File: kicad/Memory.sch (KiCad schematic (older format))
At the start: 0 parts

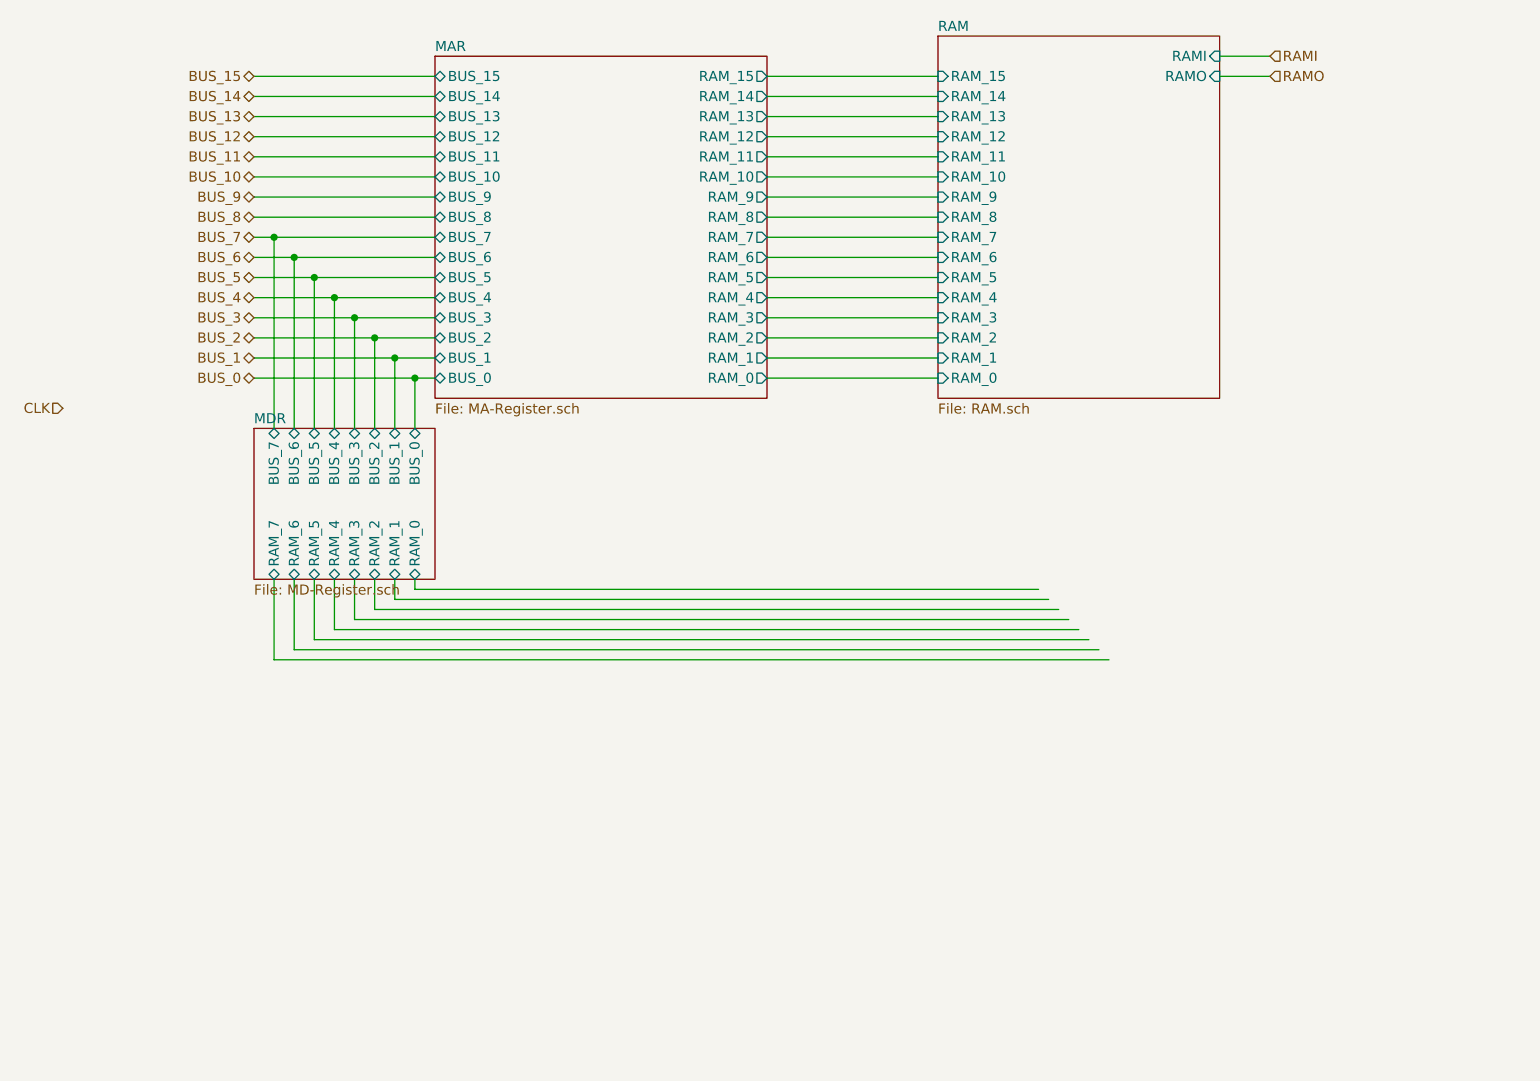
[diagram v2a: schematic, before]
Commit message: Finish todo list
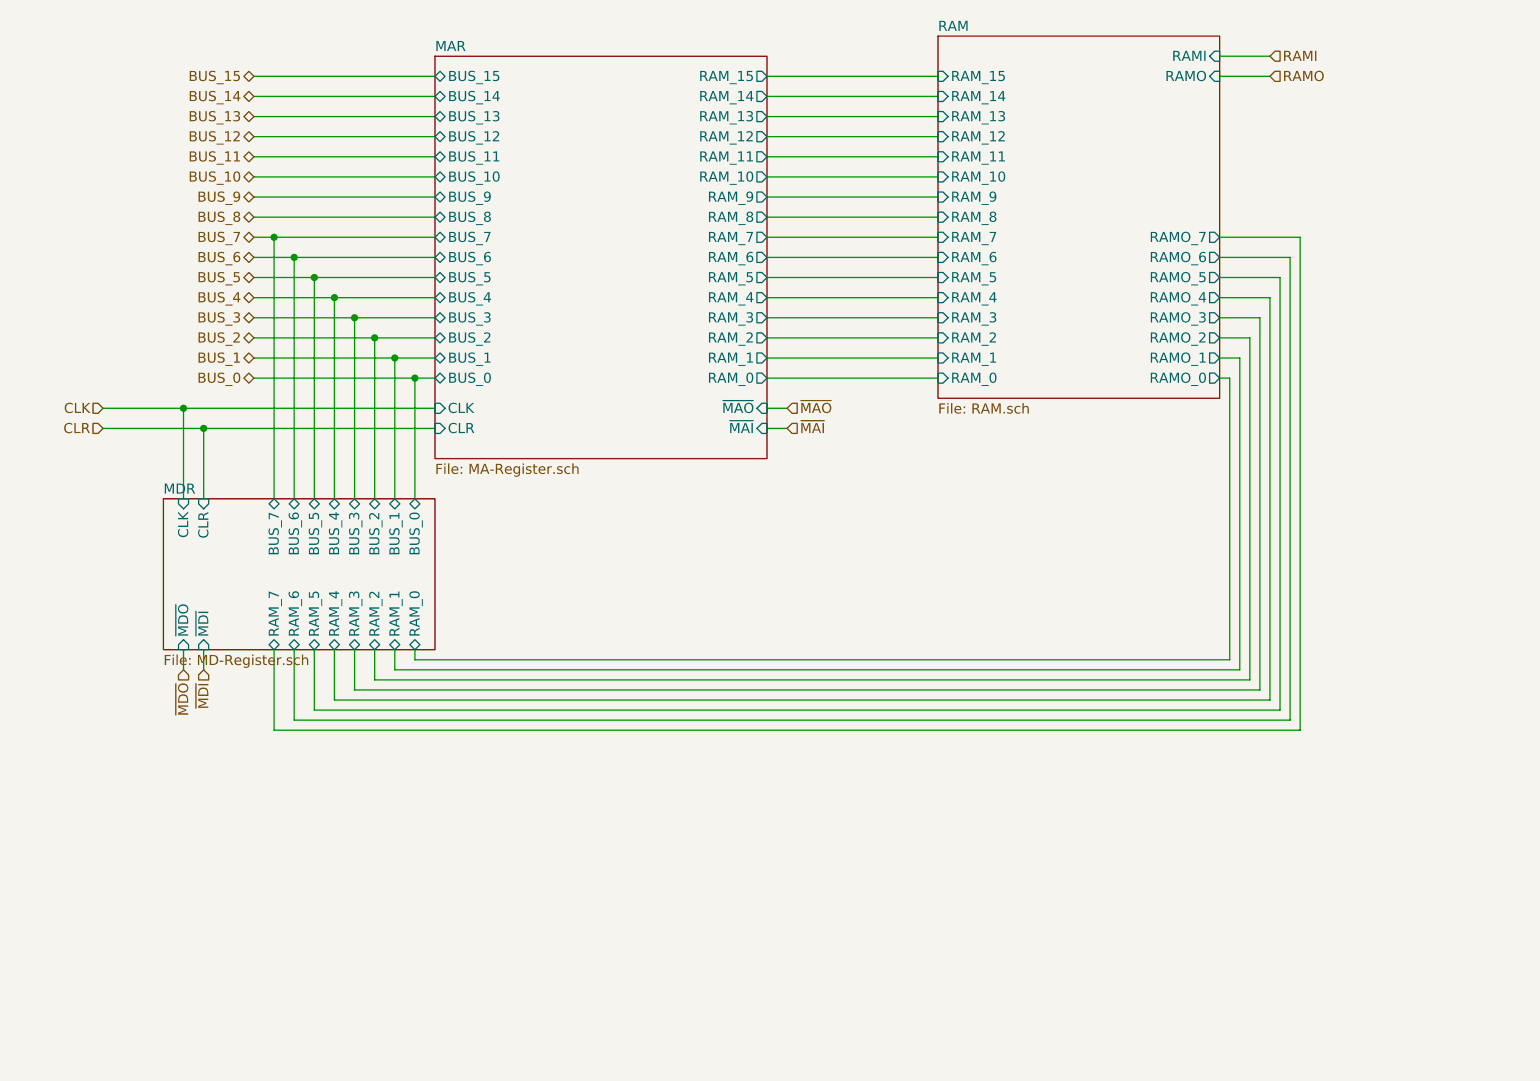
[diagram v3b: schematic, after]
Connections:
- net labels added: CLR, ~MAI~, ~MAO~, ~MDI~, ~MDO~
- wire segments 66 -> 92
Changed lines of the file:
@@
 $Descr USLetter 11000 8500
 encoding utf-8
-Sheet 13 26
+Sheet 14 26
 Title "Memory"
-Date "2019-09-26"
+Date "2019-10-03"
 Rev "v0.1"
 Comp "Christopher Milan"
@@
 Text HLabel 2050 950  0    50   BiDi ~ 0
 BUS_15
-Text HLabel 1100 2600 0    50   Input ~ 0
+Text HLabel 1300 2600 0    50   Input ~ 0
 CLK
 $Sheet
-S 2950 850  1650 1700
+S 2950 850  1650 2000
 U 5D807A05
 F0 "MAR" 50
@@
 F32 "RAM_14" O R 4600 1050 50
 F33 "RAM_15" O R 4600 950 50
+F34 "CLK" I L 2950 2600 50
+F35 "~MAO~" I R 4600 2600 50
+F36 "~MAI~" I R 4600 2700 50
+F37 "CLR" I L 2950 2700 50
 $EndSheet
 Wire Wire Line
@@
 	2050 2350 2750 2350
 Wire Wire Line
-	2850 2700 2850 2450
+	2850 3050 2850 2450
 Connection ~ 2850 2450
 Wire Wire Line
 	2850 2450 2950 2450
 Wire Wire Line
-	2750 2350 2750 2700
+	2750 2350 2750 3050
 Connection ~ 2750 2350
 Wire Wire Line
 	2750 2350 2950 2350
 Wire Wire Line
-	2650 2700 2650 2250
+	2650 3050 2650 2250
 Connection ~ 2650 2250
 Wire Wire Line
@@
 	2050 2250 2650 2250
 Wire Wire Line
-	2550 2150 2550 2700
+	2550 2150 2550 3050
 Connection ~ 2550 2150
 Wire Wire Line
 	2550 2150 2950 2150
 Wire Wire Line
-	2450 2700 2450 2050
+	2450 3050 2450 2050
 Connection ~ 2450 2050
 Wire Wire Line
 	2450 2050 2950 2050
 Wire Wire Line
-	2350 1950 2350 2700
+	2350 1950 2350 3050
 Connection ~ 2350 1950
 Wire Wire Line
 	2350 1950 2950 1950
 Wire Wire Line
-	2250 2700 2250 1850
+	2250 3050 2250 1850
 Connection ~ 2250 1850
 Wire Wire Line
 	2250 1850 2950 1850
 Wire Wire Line
-	2150 1750 2150 2700
+	2150 1750 2150 3050
 Connection ~ 2150 1750
 Wire Wire Line
 	2150 1750 2950 1750
-$Sheet
-S 2050 2700 900  750
-U 5D8079E9
-F0 "MDR" 50
-F1 "MD-Register.sch" 50
-F2 "BUS_0" B T 2850 2700 50
-F3 "BUS_1" B T 2750 2700 50
-F4 "BUS_2" B T 2650 2700 50
-F5 "BUS_3" B T 2550 2700 50
-F6 "BUS_4" B T 2450 2700 50
-F7 "BUS_5" B T 2350 2700 50
-F8 "BUS_6" B T 2250 2700 50
-F9 "BUS_7" B T 2150 2700 50
-F10 "RAM_0" B B 2850 3450 50
-F11 "RAM_1" B B 2750 3450 50
-F12 "RAM_2" B B 2650 3450 50
-F13 "RAM_3" B B 2550 3450 50
-F14 "RAM_4" T B 2450 3450 50
-F15 "RAM_5" B B 2350 3450 50
-F16 "RAM_6" B B 2250 3450 50
-F17 "RAM_7" B B 2150 3450 50
-$EndSheet
 Wire Wire Line
 	4600 1050 5450 1050
@@
 	4600 2450 5450 2450
 Wire Wire Line
-	5950 3500 2850 3500
-Wire Wire Line
-	2850 3500 2850 3450
-Wire Wire Line
-	2750 3450 2750 3550
-Wire Wire Line
-	2750 3550 6000 3550
-Wire Wire Line
-	6050 3600 2650 3600
-Wire Wire Line
-	2650 3600 2650 3450
-Wire Wire Line
-	6100 3650 2550 3650
-Wire Wire Line
-	2550 3650 2550 3450
-Wire Wire Line
-	2450 3450 2450 3700
-Wire Wire Line
-	2450 3700 6150 3700
-Wire Wire Line
-	6200 3750 2350 3750
-Wire Wire Line
-	2350 3750 2350 3450
-Wire Wire Line
-	2250 3450 2250 3800
-Wire Wire Line
-	2250 3800 6250 3800
-Wire Wire Line
-	6300 3850 2150 3850
-Wire Wire Line
-	2150 3850 2150 3450
+	2850 3850 2850 3800
+Wire Wire Line
+	2750 3800 2750 3900
+Wire Wire Line
+	2650 3950 2650 3800
+Wire Wire Line
+	2550 4000 2550 3800
+Wire Wire Line
+	2450 3800 2450 4050
+Wire Wire Line
+	2350 4100 2350 3800
+Wire Wire Line
+	2250 3800 2250 4150
+Wire Wire Line
+	2150 4200 2150 3800
 $Sheet
 S 5450 750  1400 1800
@@
 F18 "RAMI" I R 6850 850 50
 F19 "RAMO" I R 6850 950 50
+F20 "RAMO_0" O R 6850 2450 50
+F21 "RAMO_1" O R 6850 2350 50
+F22 "RAMO_2" O R 6850 2250 50
+F23 "RAMO_3" O R 6850 2150 50
+F24 "RAMO_4" O R 6850 2050 50
+F25 "RAMO_5" O R 6850 1950 50
+F26 "RAMO_6" O R 6850 1850 50
+F27 "RAMO_7" O R 6850 1750 50
 $EndSheet
 Wire Wire Line
@@
 Wire Wire Line
 	7100 950  6850 950
+Wire Wire Line
+	6850 2450 6900 2450
+Wire Wire Line
+	6900 2450 6900 3850
+Wire Wire Line
+	2850 3850 6900 3850
+Wire Wire Line
+	6950 3900 6950 2350
+Wire Wire Line
+	6950 2350 6850 2350
+Wire Wire Line
+	2750 3900 6950 3900
+Wire Wire Line
+	6850 2250 7000 2250
+Wire Wire Line
+	7000 2250 7000 3950
+Wire Wire Line
+	2650 3950 7000 3950
+Wire Wire Line
+	7050 4000 7050 2150
+Wire Wire Line
+	7050 2150 6850 2150
+Wire Wire Line
+	2550 4000 7050 4000
+Wire Wire Line
+	6850 2050 7100 2050
+Wire Wire Line
+	7100 2050 7100 4050
+Wire Wire Line
+	2450 4050 7100 4050
+Wire Wire Line
+	7150 4100 7150 1950
+Wire Wire Line
+	7150 1950 6850 1950
+Wire Wire Line
+	2350 4100 7150 4100
+Wire Wire Line
+	6850 1850 7200 1850
+Wire Wire Line
+	7200 1850 7200 4150
+Wire Wire Line
+	2250 4150 7200 4150
+Wire Wire Line
+	7250 4200 7250 1750
+Wire Wire Line
+	7250 1750 6850 1750
+Wire Wire Line
+	2150 4200 7250 4200
+Wire Wire Line
+	1300 2600 1700 2600
+Wire Wire Line
+	1700 2600 1700 3050
+Text HLabel 1800 3900 3    50   Input ~ 0
+~MDI~
+Text HLabel 1700 3900 3    50   Input ~ 0
+~MDO~
+Wire Wire Line
+	1700 3900 1700 3800
+Wire Wire Line
+	1800 3900 1800 3800
+$Sheet
+S 1600 3050 1350 750
+U 5D8079E9
+F0 "MDR" 50
+F1 "MD-Register.sch" 50
+F2 "BUS_0" B T 2850 3050 50
+F3 "BUS_1" B T 2750 3050 50
+F4 "BUS_2" B T 2650 3050 50
+F5 "BUS_3" B T 2550 3050 50
+F6 "BUS_4" B T 2450 3050 50
+F7 "BUS_5" B T 2350 3050 50
+F8 "BUS_6" B T 2250 3050 50
+F9 "BUS_7" B T 2150 3050 50
+F10 "RAM_0" B B 2850 3800 50
+F11 "RAM_1" B B 2750 3800 50
+F12 "RAM_2" B B 2650 3800 50
+F13 "RAM_3" B B 2550 3800 50
+F14 "RAM_4" T B 2450 3800 50
+F15 "RAM_5" B B 2350 3800 50
+F16 "RAM_6" B B 2250 3800 50
+F17 "RAM_7" B B 2150 3800 50
+F18 "CLK" I T 1700 3050 50
+F19 "~MDO~" I B 1700 3800 50
+F20 "~MDI~" I B 1800 3800 50
+F21 "CLR" I T 1800 3050 50
+$EndSheet
+Text HLabel 1300 2700 0    50   Input ~ 0
+CLR
+Wire Wire Line
+	1300 2700 1800 2700
+Wire Wire Line
+	1800 2700 1800 3050
+Wire Wire Line
+	1800 2700 2950 2700
+Connection ~ 1800 2700
+Wire Wire Line
+	2950 2600 1700 2600
+Connection ~ 1700 2600
+Text HLabel 4700 2700 2    50   Input ~ 0
+~MAI~
+Text HLabel 4700 2600 2    50   Input ~ 0
+~MAO~
+Wire Wire Line
+	4700 2700 4600 2700
+Wire Wire Line
+	4700 2600 4600 2600
 $EndSCHEMATC

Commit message: Up to v1.0 and plot
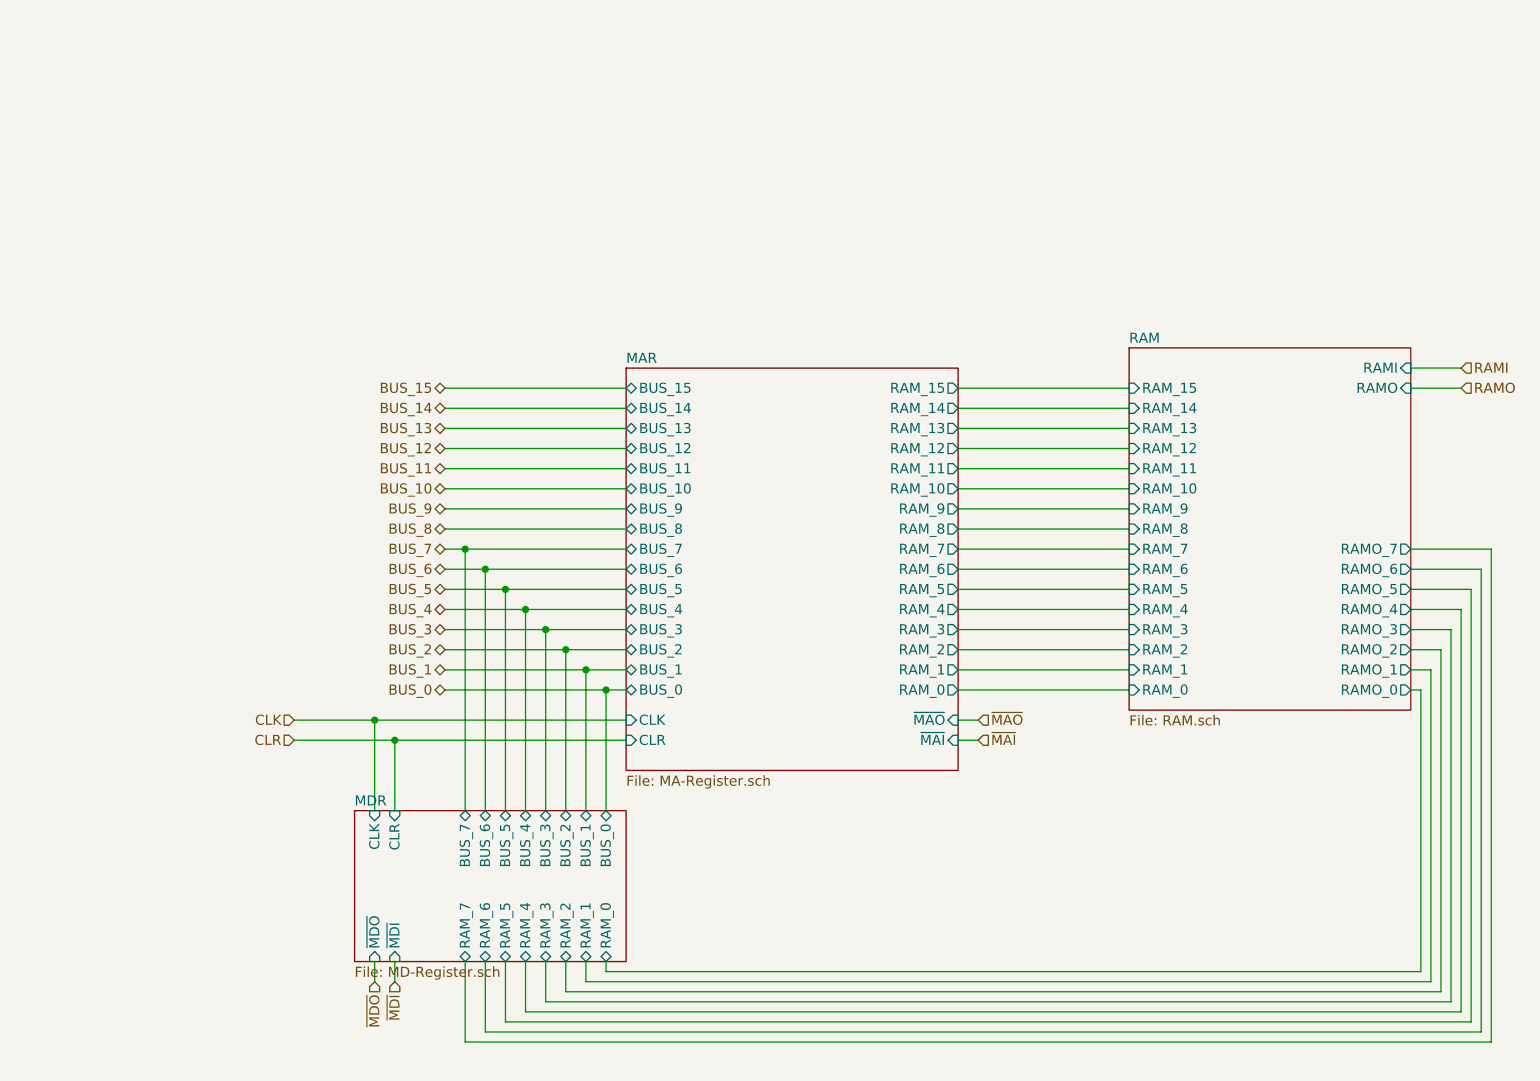
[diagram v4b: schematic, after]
